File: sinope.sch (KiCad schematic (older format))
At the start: 46 parts, among them J1 PIOA, J2 SERIAL0, J3 PIOB, J4 SERIAL1, J5 Battery, J6 5VDC, Q1 3N3906, SW1 RESET, U1 Z80CPU, U10 MEMORY_GAL, U11 74LS157, U12 TC551001, U2 Z80CTC, U3 Z80PIO, U4 Z80SIO, U5 MAX232, U6 MAX232, U7 IO_GAL, U8 MAX695, U9 27C010, X1 3.6864Mhz

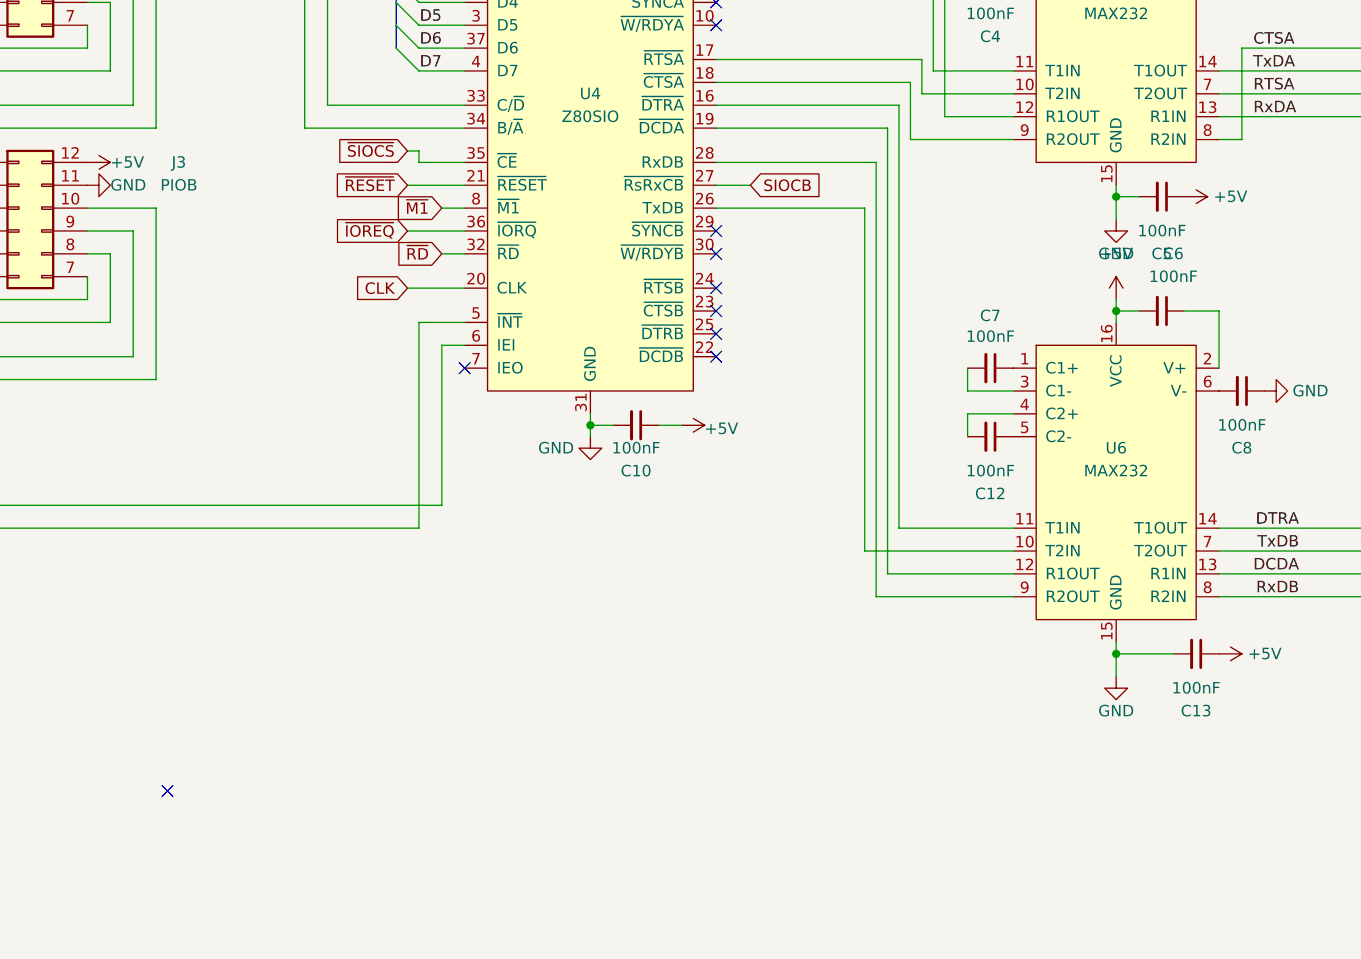
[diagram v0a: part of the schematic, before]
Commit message: Package assignments, PCB work
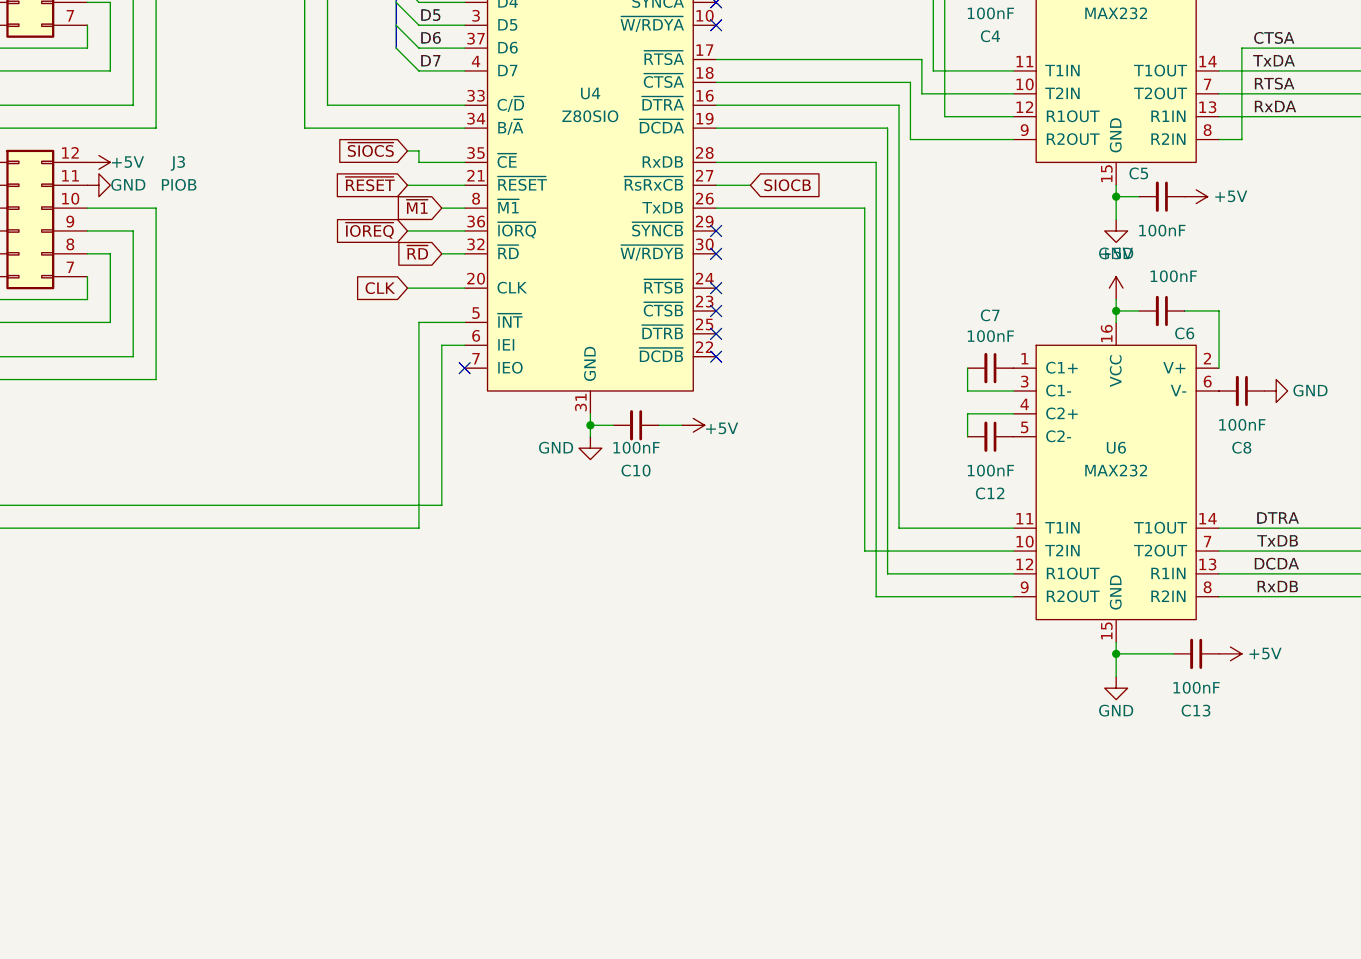
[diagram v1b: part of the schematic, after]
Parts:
- U10, U7: footprint (none) -> Package_DIP:DIP-24_W7.62mm
- U11: footprint (none) -> Package_DIP:DIP-16_W7.62mm
- U9: footprint (none) -> Package_DIP:DIP-32_W15.24mm
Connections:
- no-connect marks 38 -> 37
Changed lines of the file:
@@
 U 1 1 5F7E8ED7
 P 13750 2950
-F 0 "C6" V 13500 3000 50  0000 C CNN
+F 0 "C6" V 13850 3050 50  0000 C CNN
 F 1 "100nF" V 13600 3000 50  0000 C CNN
 F 2 "Capacitor_SMD:C_0805_2012Metric" H 13750 2950 50  0001 C CNN
@@
 U 1 1 5F76B641
 P 13750 2450
-F 0 "C5" V 14000 2450 50  0000 C CNN
+F 0 "C5" V 13650 2350 50  0000 C CNN
 F 1 "100nF" V 13900 2450 50  0000 C CNN
 F 2 "Capacitor_SMD:C_0805_2012Metric" H 13750 2450 50  0001 C CNN
@@
 F 0 "U11" H 11000 8250 50  0000 C CNN
 F 1 "74LS157" H 11100 8150 50  0000 C CNN
-F 2 "" H 11000 8250 50  0001 C CNN
+F 2 "Package_DIP:DIP-16_W7.62mm" H 11000 8250 50  0001 C CNN
 F 3 "http://www.ti.com/lit/gpn/sn74LS157" H 11000 8250 50  0001 C CNN
 	1    11000 8400
@@
 F 0 "U9" H 7000 7400 50  0000 C CNN
 F 1 "27C010" H 7000 7300 50  0000 C CNN
-F 2 "" H 6900 7750 50  0001 C CNN
+F 2 "Package_DIP:DIP-32_W15.24mm" H 6900 7750 50  0001 C CNN
 F 3 "http://ww1.microchip.com/downloads/en/DeviceDoc/doc0321.pdf" H 6900 7750 50  0001 C CNN
 	1    6900 7750
@@
 	3650 6250 6200 6250
 NoConn ~ 3700 8750
-NoConn ~ 9400 5050
 Wire Wire Line
 	10150 9400 10250 9500
@@
 F 0 "U10" H 9150 8700 50  0000 C CNN
 F 1 "MEMORY_GAL" H 9150 8600 50  0000 C CNN
-F 2 "" H 9050 8900 50  0001 C CNN
+F 2 "Package_DIP:DIP-24_W7.62mm" H 9050 8900 50  0001 C CNN
 F 3 "" H 9050 8900 50  0001 C CNN
 	1    9100 8900
@@
 F 0 "U7" H 4950 5000 50  0000 C CNN
 F 1 "IO_GAL" H 5000 4900 50  0000 C CNN
-F 2 "" H 4900 5100 50  0001 C CNN
+F 2 "Package_DIP:DIP-24_W7.62mm" H 4900 5100 50  0001 C CNN
 F 3 "" H 4900 5100 50  0001 C CNN
 	1    4900 5100
